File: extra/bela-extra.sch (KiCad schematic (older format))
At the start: 20 parts

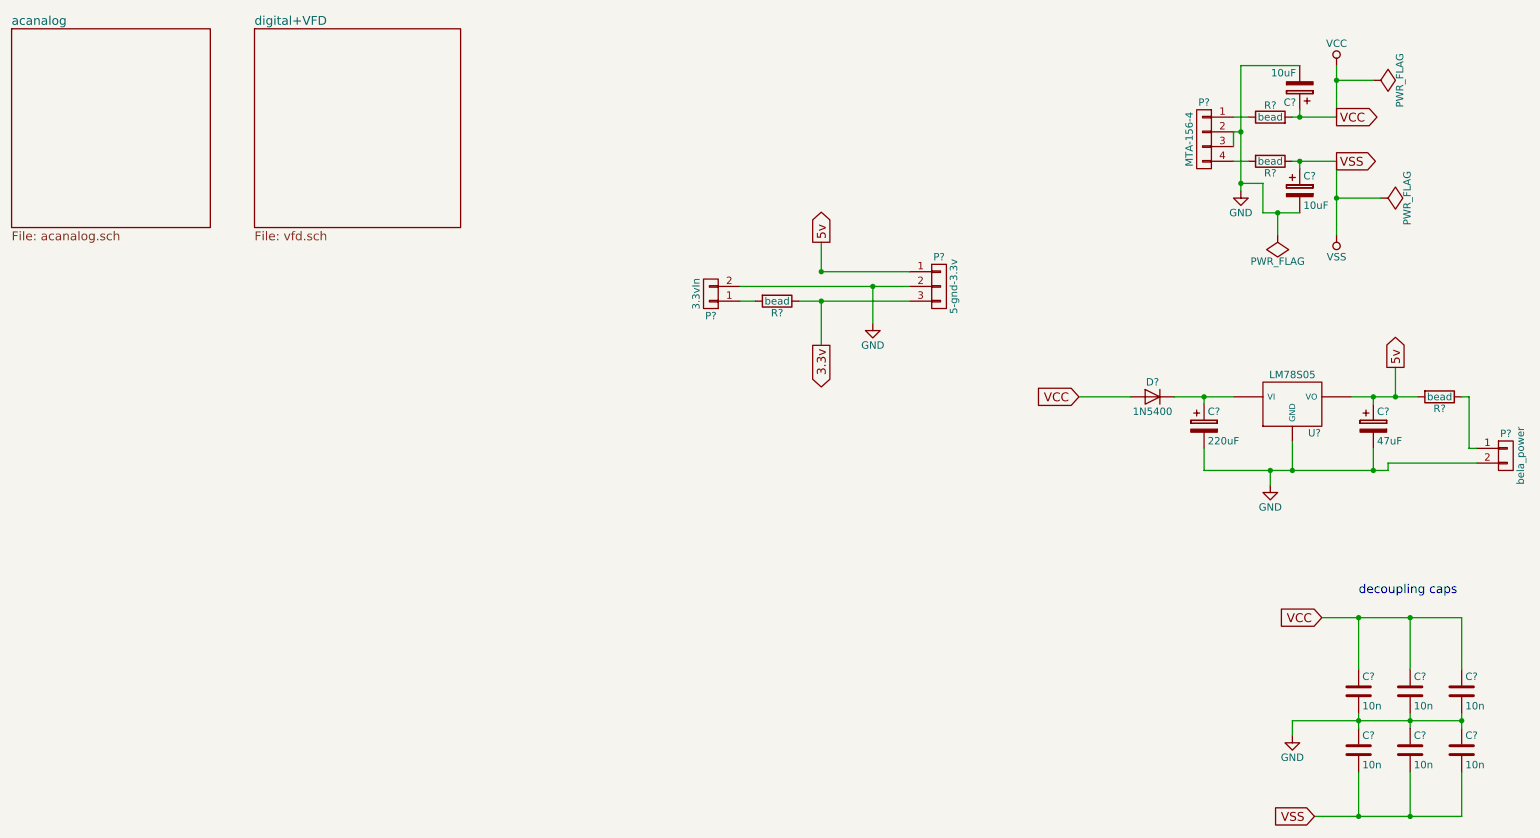
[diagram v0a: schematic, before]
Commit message: a bunch more hooking up
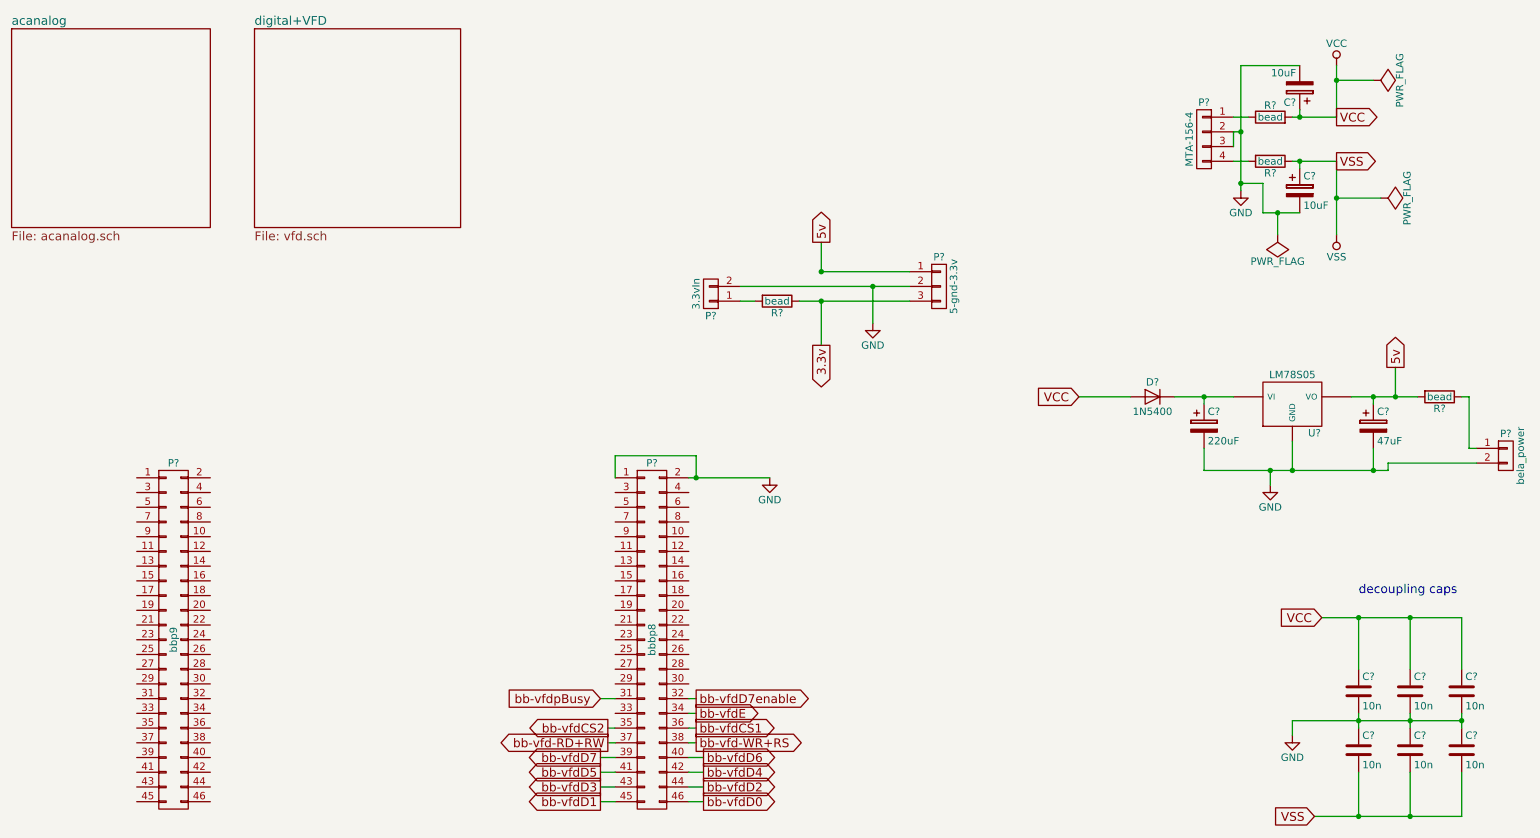
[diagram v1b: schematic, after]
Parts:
- added P?: bbp9, symbol CONN_02X23
- added P?: bbbp8, symbol CONN_02X23
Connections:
- net GND: now also P?.1 (P1), P?.2 (P2)
- new net bb-vfd-RD+RW: P?.37 (P37)
- new net bb-vfd-WR+RS: P?.38 (P38)
- new net bb-vfdCS1: P?.36 (P36)
- new net bb-vfdCS2: P?.35 (P35)
- new net bb-vfdD0: P?.46 (P46)
- new net bb-vfdD1: P?.45 (P45)
- new net bb-vfdD2: P?.44 (P44)
- new net bb-vfdD3: P?.43 (P43)
- new net bb-vfdD4: P?.42 (P42)
- new net bb-vfdD5: P?.41 (P41)
- new net bb-vfdD6: P?.40 (P40)
- new net bb-vfdD7: P?.39 (P39)
- new net bb-vfdD7enable: P?.32 (P32)
- new net bb-vfdE: P?.34 (P34)
- new net bb-vfdpBusy: P?.31 (P31)
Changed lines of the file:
@@
 $EndComp
 Wire Wire Line
-	6750 2400 5600 2400
+	5600 2400 6750 2400
 Text GLabel 6150 2100 1    60   Output ~ 0
 5v
@@
 Wire Wire Line
 	6150 2300 6750 2300
+$Comp
+L CONN_02X23 P?
+U 1 1 586B0458
+P 1750 4800
+F 0 "P?" H 1750 6000 50  0000 C CNN
+F 1 "bbp9" V 1750 4800 50  0000 C CNN
+F 2 "" H 1750 3950 50  0000 C CNN
+F 3 "" H 1750 3950 50  0000 C CNN
+	1    1750 4800
+	1    0    0    -1
+$EndComp
+$Comp
+L CONN_02X23 P?
+U 1 1 586B04DD
+P 5000 4800
+F 0 "P?" H 5000 6000 50  0000 C CNN
+F 1 "bbbp8" V 5000 4800 50  0000 C CNN
+F 2 "" H 5000 3950 50  0000 C CNN
+F 3 "" H 5000 3950 50  0000 C CNN
+	1    5000 4800
+	1    0    0    -1
+$EndComp
+$Comp
+L GND #PWR?
+U 1 1 586B08A6
+P 5800 3700
+F 0 "#PWR?" H 5800 3450 50  0001 C CNN
+F 1 "GND" H 5800 3550 50  0000 C CNN
+F 2 "" H 5800 3700 50  0000 C CNN
+F 3 "" H 5800 3700 50  0000 C CNN
+	1    5800 3700
+	1    0    0    -1
+$EndComp
+Wire Wire Line
+	5250 3700 5800 3700
+Wire Wire Line
+	4750 3700 4750 3550
+Wire Wire Line
+	4750 3550 5300 3550
+Wire Wire Line
+	5300 3550 5300 3700
+Connection ~ 5300 3700
+Text GLabel 5300 5200 2    60   Output ~ 0
+bb-vfdD7enable
+Text GLabel 5350 5900 2    60   Output ~ 0
+bb-vfdD0
+Text GLabel 4650 5900 0    60   Output ~ 0
+bb-vfdD1
+Text GLabel 5350 5800 2    60   Output ~ 0
+bb-vfdD2
+Text GLabel 4650 5800 0    60   Output ~ 0
+bb-vfdD3
+Text GLabel 5350 5700 2    60   Output ~ 0
+bb-vfdD4
+Text GLabel 4650 5700 0    60   Output ~ 0
+bb-vfdD5
+Text GLabel 5350 5600 2    60   Output ~ 0
+bb-vfdD6
+Text GLabel 4650 5600 0    60   Output ~ 0
+bb-vfdD7
+Wire Wire Line
+	5250 5900 5350 5900
+Wire Wire Line
+	5350 5800 5250 5800
+Wire Wire Line
+	5250 5700 5350 5700
+Wire Wire Line
+	5250 5600 5350 5600
+Wire Wire Line
+	4750 5600 4650 5600
+Wire Wire Line
+	4650 5700 4750 5700
+Wire Wire Line
+	4750 5800 4650 5800
+Wire Wire Line
+	4650 5900 4750 5900
+Text GLabel 5300 5500 2    60   Output ~ 0
+bb-vfd-WR+RS
+Text GLabel 4700 5500 0    60   Output ~ 0
+bb-vfd-RD+RW
+Text GLabel 5300 5400 2    60   Output ~ 0
+bb-vfdCS1
+Text GLabel 4700 5400 0    60   Output ~ 0
+bb-vfdCS2
+Wire Wire Line
+	4750 5500 4700 5500
+Wire Wire Line
+	5250 5500 5300 5500
+Wire Wire Line
+	4750 5400 4700 5400
+Wire Wire Line
+	5250 5400 5300 5400
+Text GLabel 5300 5300 2    60   Output ~ 0
+bb-vfdE
+Wire Wire Line
+	5300 5300 5250 5300
+Text GLabel 4650 5200 0    60   Input ~ 0
+bb-vfdpBusy
+Wire Wire Line
+	5250 5200 5300 5200
+Wire Wire Line
+	4650 5200 4750 5200
 $EndSCHEMATC
